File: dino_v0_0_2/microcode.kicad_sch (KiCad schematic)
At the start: 4 parts, among them U15 AT28C64B, U16 74LS244N, U17 74LS244N, U9 AT28C64B

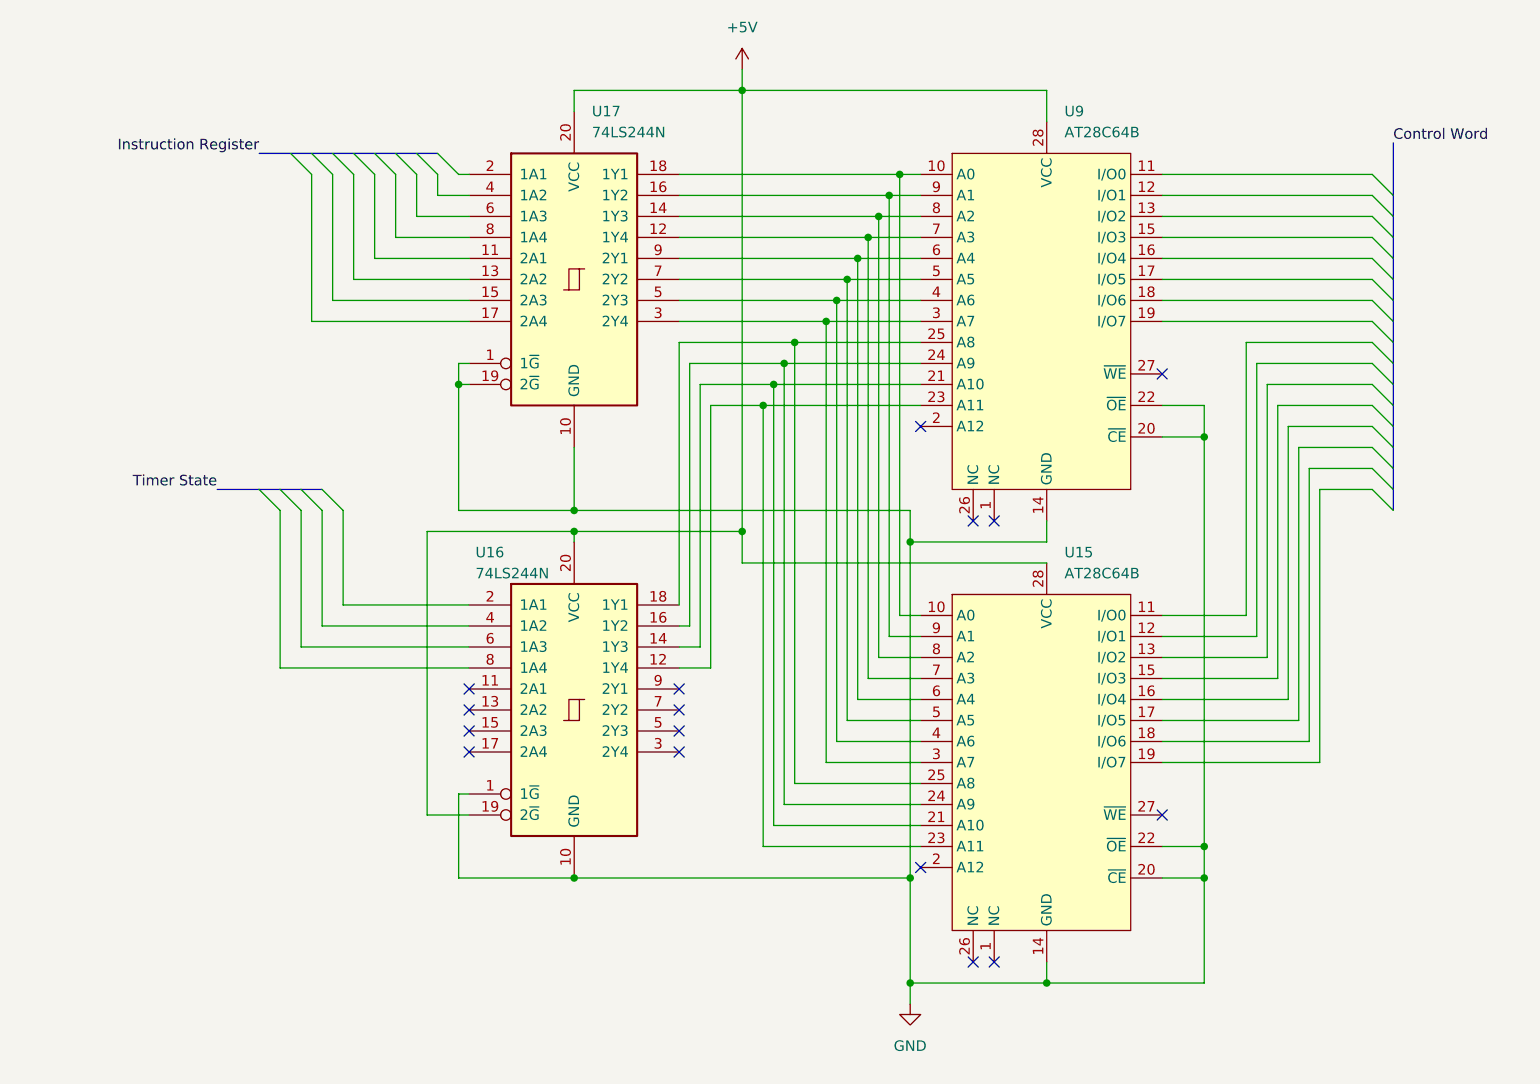
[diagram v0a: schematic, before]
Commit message: Update
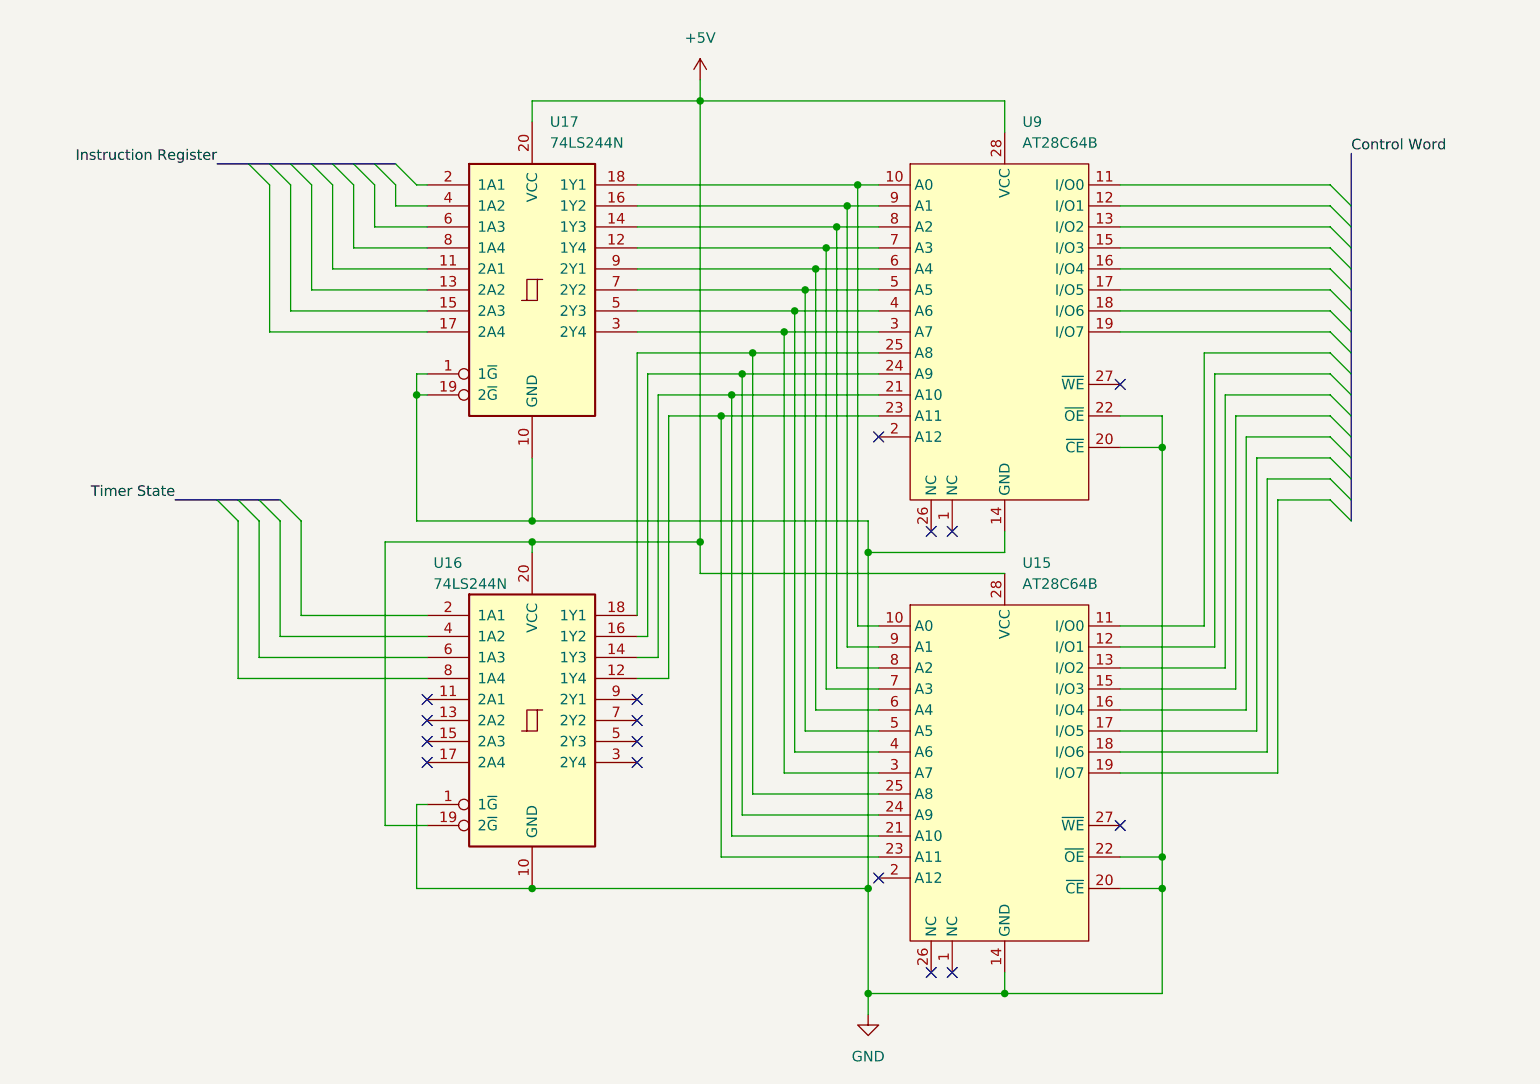
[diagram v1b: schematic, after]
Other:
- moved on the sheet: U15, U16, U17, U9
